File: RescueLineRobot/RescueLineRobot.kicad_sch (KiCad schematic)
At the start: 8 parts, among them J1 Conn_01x11, J2 Bateria, J3 Motor 1, J4 Motor 2, J5 Convertidor, U1 ROB-14450, U2 ESP32-DEVKIT-V1

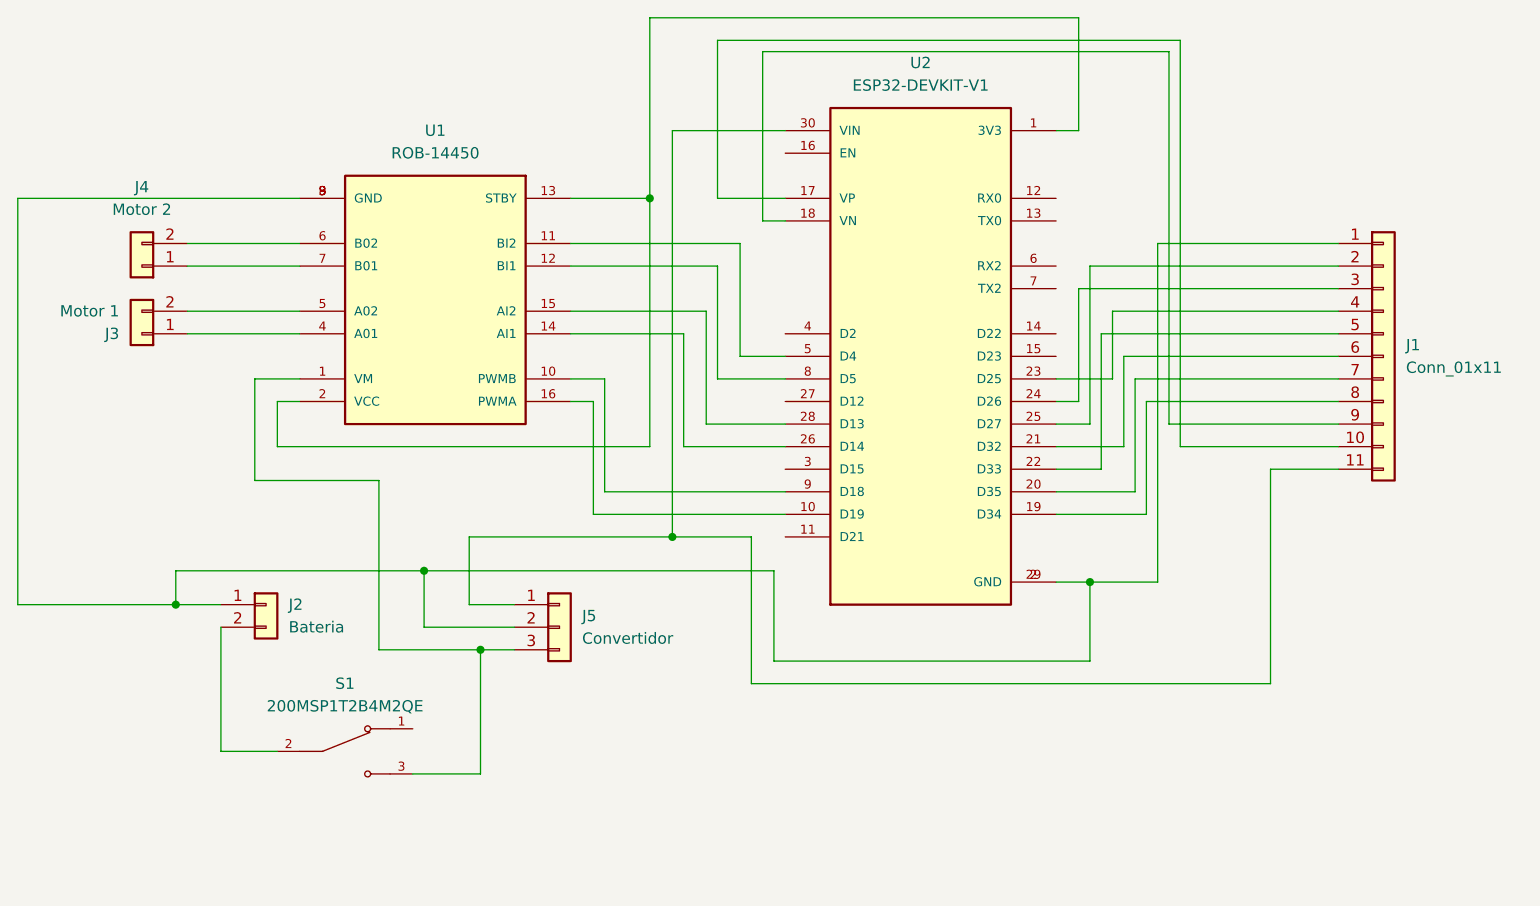
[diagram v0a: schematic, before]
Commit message: updates
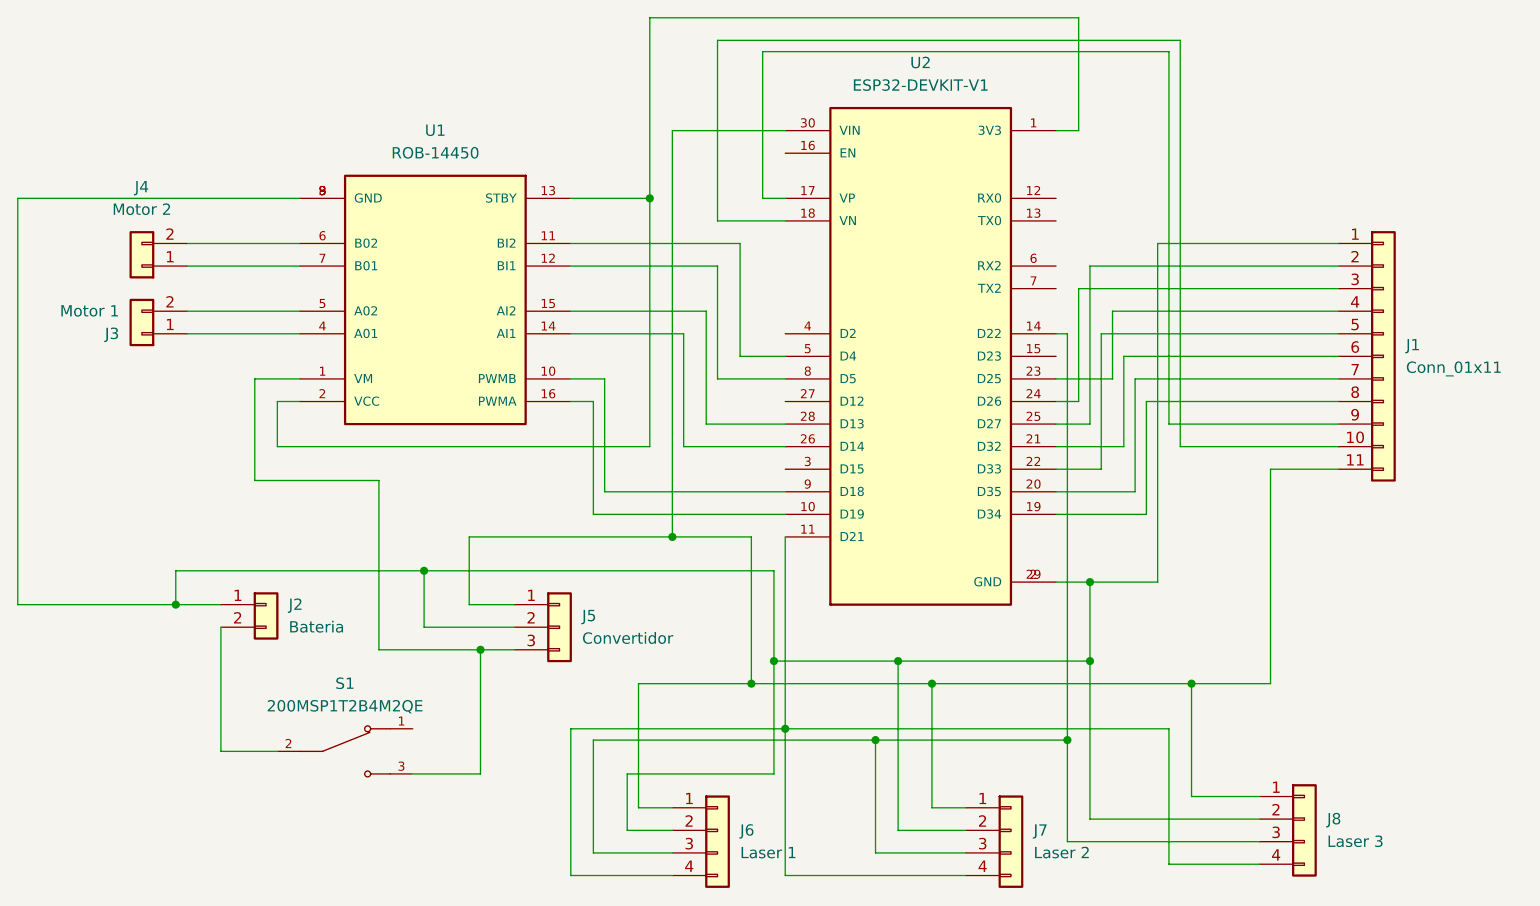
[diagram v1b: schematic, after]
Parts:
- added J6: Laser 1, Connector_JST:JST_XH_B4B-XH-A_1x04_P2.50mm_Vertical, symbol Connector_Generic:Conn_01x04
- added J7: Laser 2, Connector_JST:JST_XH_B4B-XH-A_1x04_P2.50mm_Vertical, symbol Connector_Generic:Conn_01x04
- added J8: Laser 3, Connector_JST:JST_XH_B4B-XH-A_1x04_P2.50mm_Vertical, symbol Connector_Generic:Conn_01x04
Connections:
- net at J1.1 (Pin_1), J2.1 (Pin_1), J5.2 (Pin_2)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: now also J6.2 (Pin_2), J7.2 (Pin_2), J8.2 (Pin_2)
- net at J1.11 (Pin_11), J5.1 (Pin_1), U2.30 (VIN): now also J6.1 (Pin_1), J7.1 (Pin_1), J8.1 (Pin_1)
- net at U2.11 (D21): now also J6.4 (Pin_4), J7.4 (Pin_4), J8.4 (Pin_4)
- net at U2.14 (D22): now also J6.3 (Pin_3), J7.3 (Pin_3), J8.3 (Pin_3)
- net at U2.17 (VP): now also J1.9 (Pin_9); no longer J1.10 (Pin_10)
- net at U2.18 (VN): now also J1.10 (Pin_10); no longer J1.9 (Pin_9)
